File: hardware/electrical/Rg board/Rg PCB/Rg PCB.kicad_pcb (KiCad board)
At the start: 2 copper layers, 19.7 x 26.2 mm, 10 parts, among them J1 Conn_01x03, J2 Conn_01x01_Pin

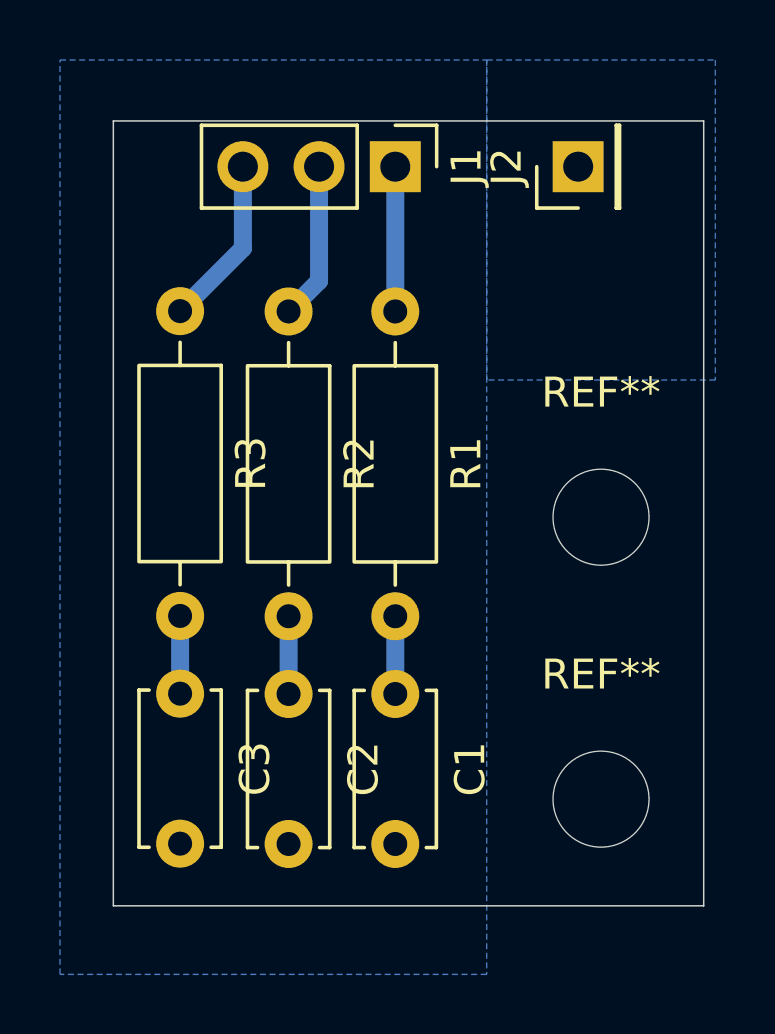
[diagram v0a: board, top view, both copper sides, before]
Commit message: update fw readme
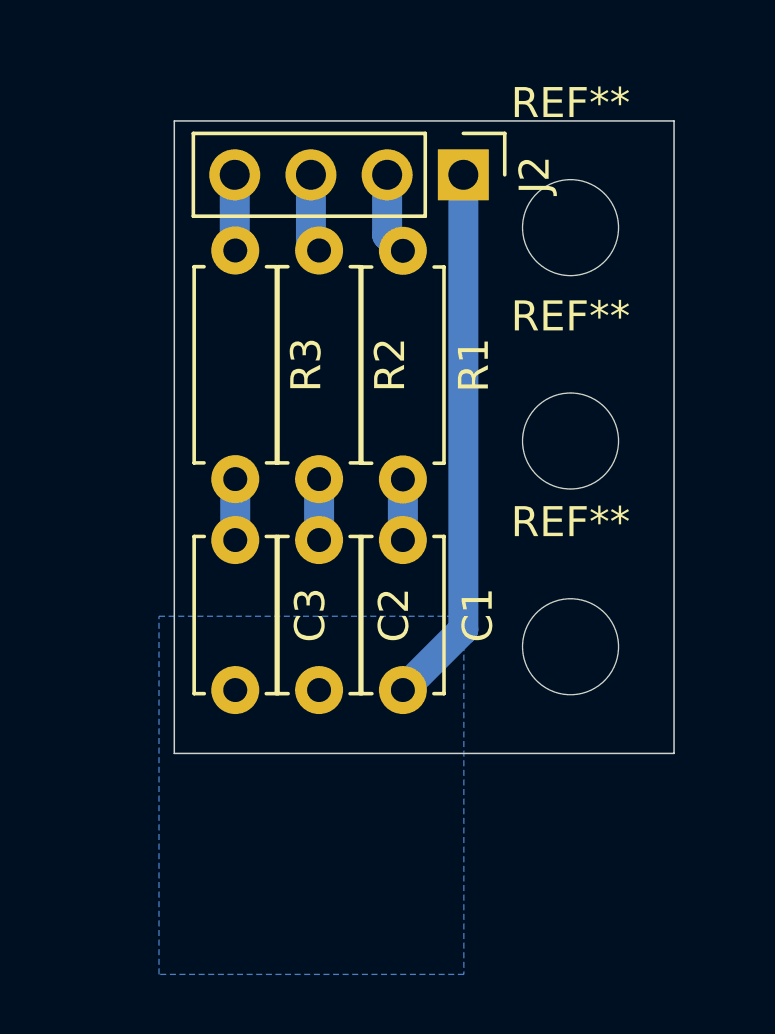
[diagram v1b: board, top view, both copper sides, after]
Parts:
- removed J1: Conn_01x03, Connector_PinHeader_2.54mm:PinHeader_1x03_P2.54mm_Vertical
- removed the REF** at (160.0, 94.5)
- added REF**: MountingHole_3.2mm_M3, MountingHole:MountingHole_3.2mm_M3, F.Cu at (159.0, 84.8)
- added REF**: MountingHole_3.2mm_M3, MountingHole:MountingHole_3.2mm_M3, F.Cu at (159.0, 91.9)
- J2: value Conn_01x01_Pin -> Conn_01x04; footprint Connector_PinHeader_2.54mm:PinHeader_1x01_P2.54mm_Vertical -> Connector_PinHeader_2.54mm:PinHeader_1x04_P2.54mm_Vertical
- R1, R2, R3: footprint Resistor_THT:R_Axial_DIN0207_L6.3mm_D2.5mm_P10.16mm_Horizontal -> Resistor_THT:R_Axial_DIN0207_L6.3mm_D2.5mm_P7.62mm_Horizontal
- moved C3 5.44 mm to (147.8, 95.2)
- moved C2 5.23 mm to (150.6, 95.2)
- moved REF** 5.18 mm to (159.0, 98.8)
- moved C1 5.14 mm to (153.4, 95.2)
- moved J2 3.84 mm to (155.4, 83.1), turned to -90 degrees
- moved R3 2.73 mm to (147.8, 85.6)
- moved R2 2.27 mm to (150.6, 85.6)
- moved R1 2.04 mm to (153.4, 85.6)
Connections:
- R1 pad 1: Net-(J1-Pin_1) -> Net-(J2-Pin_2)
- R2 pad 1: Net-(J1-Pin_2) -> Net-(J2-Pin_3)
- R3 pad 1: Net-(J1-Pin_3) -> Net-(J2-Pin_4)
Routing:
- net GND: track 0.02 -> 18.0 mm
- net Net-(J1-Pin_3): track 5.68 -> 0.00 mm
- net Net-(J1-Pin_2): track 5.25 -> 0.00 mm
- net Net-(J1-Pin_1): track 4.83 -> 0.00 mm
- net Net-(J2-Pin_2): track 0.00 -> 3.11 mm
- net Net-(J2-Pin_4): track 0.00 -> 2.89 mm
- net Net-(J2-Pin_3): track 0.00 -> 2.64 mm
- net Net-(C1-Pad1): track 2.59 -> 2.02 mm
- net Net-(C3-Pad1): track 2.59 -> 2.03 mm
- net Net-(C2-Pad1): track 2.59 -> 2.03 mm
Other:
- board size 19.7 x 26.2 mm -> 16.7 x 21.1 mm
